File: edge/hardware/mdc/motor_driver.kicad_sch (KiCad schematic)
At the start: 10 parts, among them J1 Conn_01x06, Q1 2N7000, Q2 2N7000, Q3 2N7000, Q4 2N7000, U5 74HC04

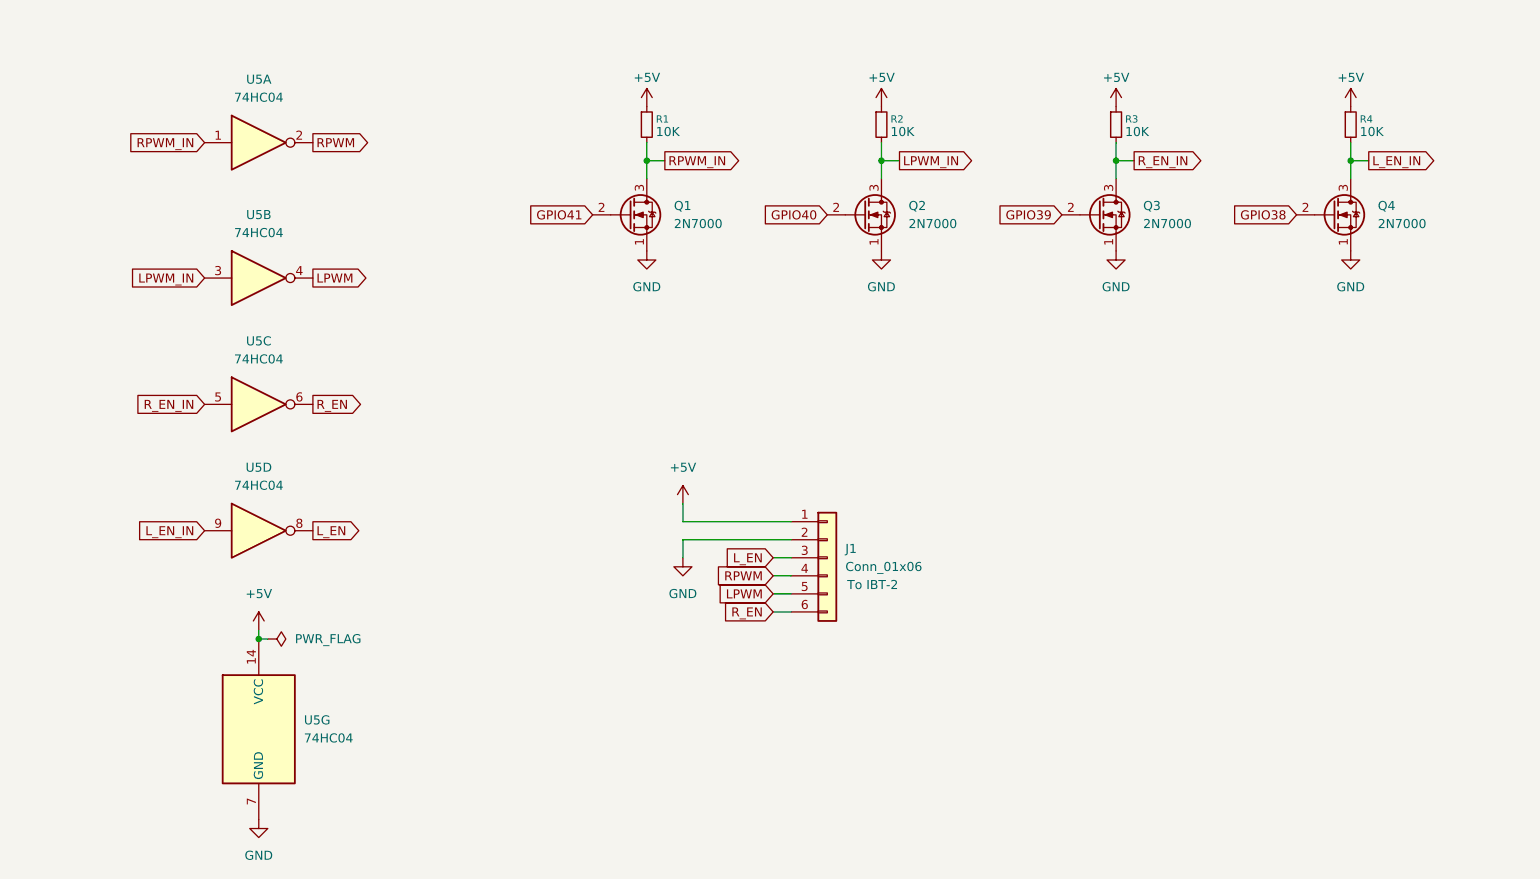
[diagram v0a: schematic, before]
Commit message: rev3.0 schematics
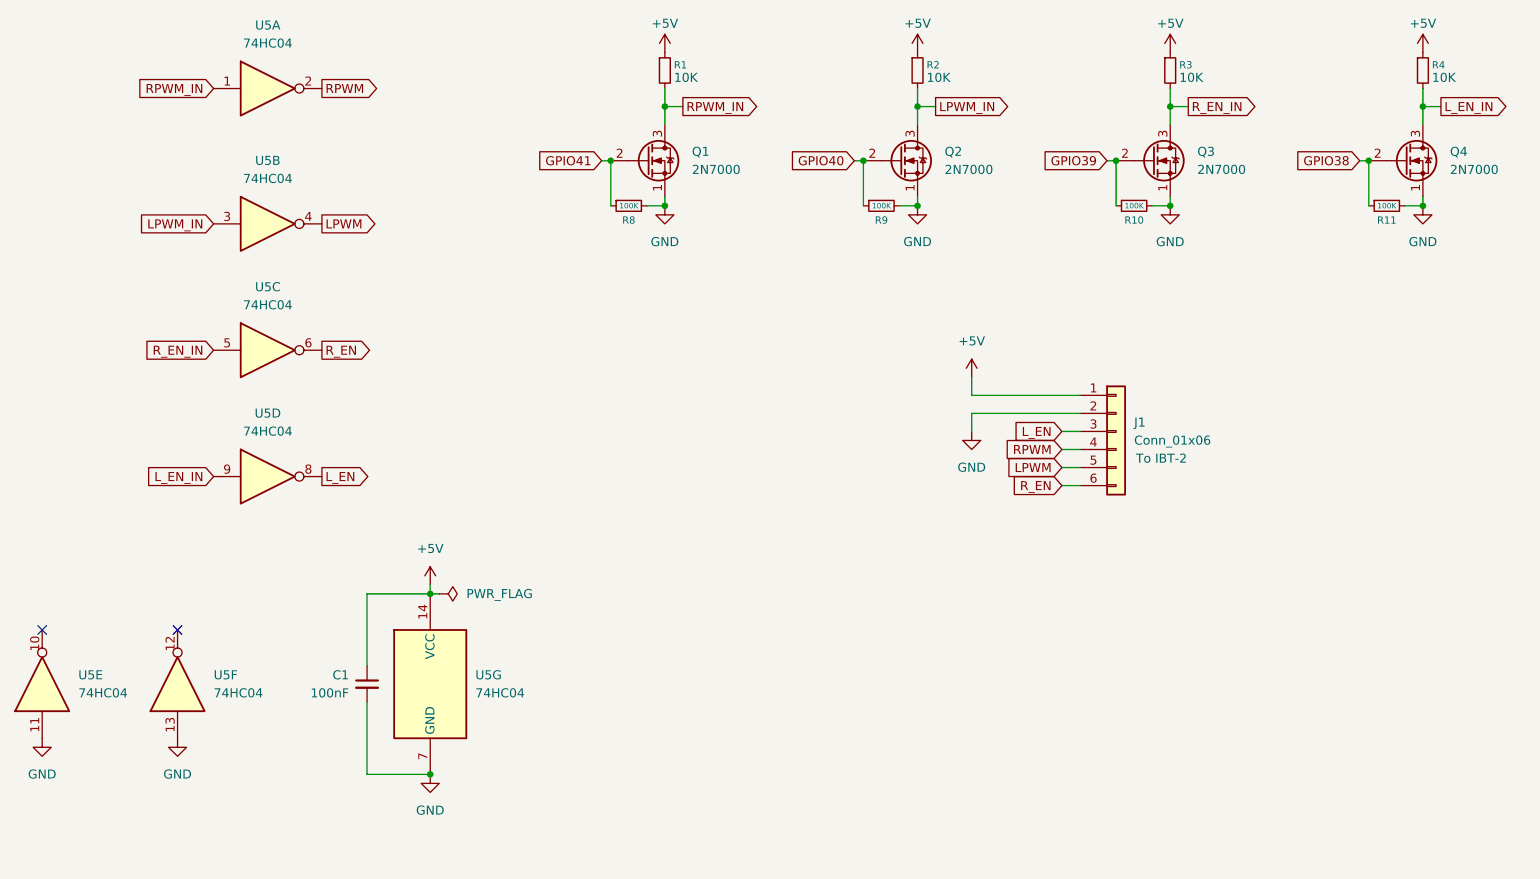
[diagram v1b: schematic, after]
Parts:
- added C1: 100nF, symbol Device:C_Small
- added R10, R11, R8, R9: 100K, symbol Device:R_Small
- added unit 5 of U5
- added unit 6 of U5
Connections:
- net +5V: now also C1.1
- net GND: now also C1.2, R10.2, R11.2, R8.2, R9.2, U5.11, U5.13
- net GPIO38: now also R11.1
- net GPIO39: now also R10.1
- net GPIO40: now also R9.1
- net GPIO41: now also R8.1
- no-connect marks 0 -> 2
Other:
- moved on the sheet: J1, Q1, Q2, Q3, Q4, R1, R2, R3, R4, U5A, U5B, U5C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
